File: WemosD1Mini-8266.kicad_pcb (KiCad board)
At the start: 2 copper layers, 79.9 x 51.8 mm, 54 parts, among them J1 Conn_01x02_Pin, J2 Screw_Terminal_01x10, J3 Conn_01x02_Pin, U1 PC817, U2 PC817, U3 PC817, U4 PC817, U5 WeMos_D1_mini, U6 ULN2003

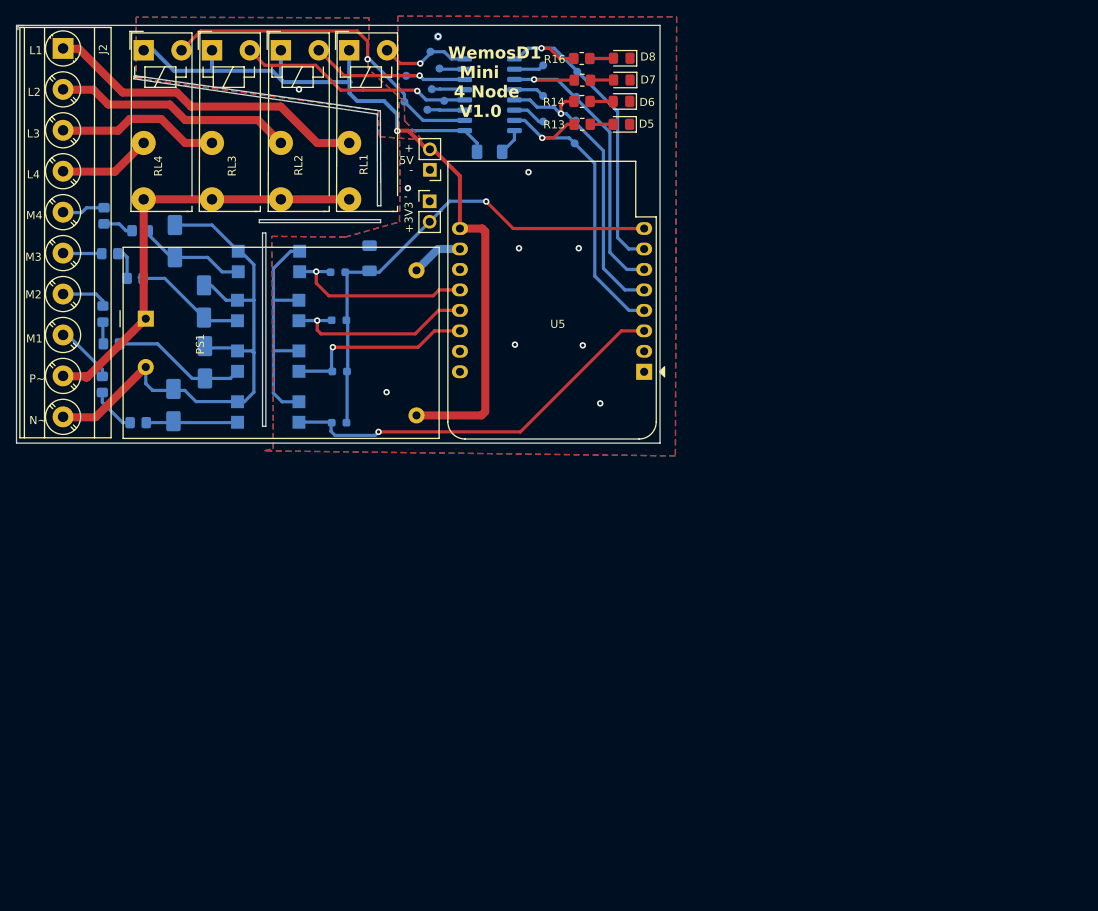
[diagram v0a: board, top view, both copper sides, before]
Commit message: Version 1.1
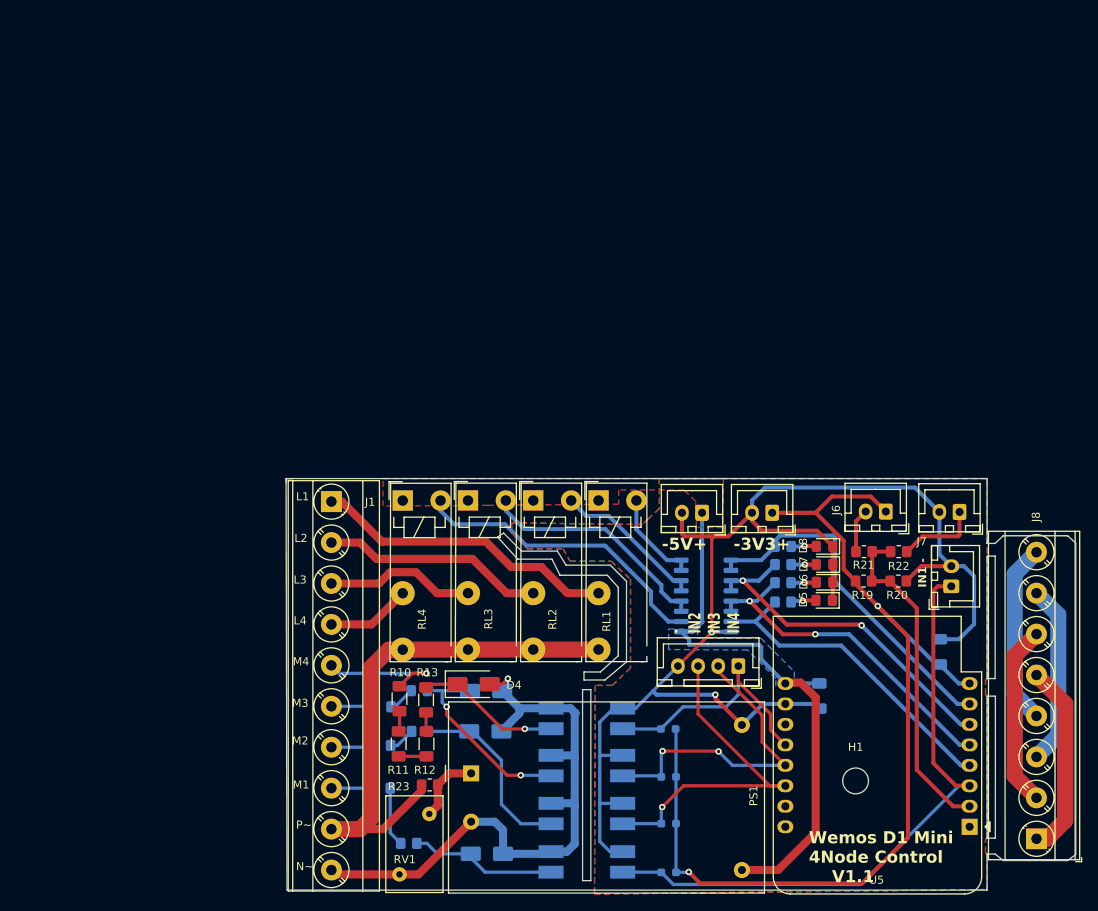
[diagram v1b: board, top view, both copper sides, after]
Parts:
- removed IJ1, IJ2, IJ3, IJ4, NCI1, NCI2, NCI3, NCR1, NCR2, NCR3, RJ1, RJ2, RJ3, RJ4: TestPoint, TestPoint:TestPoint_Pad_D1.0mm
- added H1: MountingHole, MountingHole:MountingHole_3.2mm_M3, F.Cu at (170.7, 137.5)
- added J4: Conn_01x04_Pin, Connector_JST:JST_XH_B4B-XH-A_1x04_P2.50mm_Vertical, F.Cu at (156.1, 123.3)
- added J5: Conn_01x02_Pin, Connector_JST:JST_XH_B2B-XH-A_1x02_P2.50mm_Vertical, F.Cu at (182.6, 113.4)
- added J6: Conn_01x02_Pin, Connector_JST:JST_XH_B2B-XH-A_1x02_P2.50mm_Vertical, F.Cu at (174.4, 104.1)
- added J7: Conn_01x02_Pin, Connector_JST:JST_XH_B2B-XH-A_1x02_P2.50mm_Vertical, F.Cu at (183.6, 104.1)
- added J8: Screw_Terminal_01x08, TerminalBlock_Phoenix:TerminalBlock_Phoenix_MKDS-3-8-5.08_1x08_P5.08mm_Horizontal, F.Cu at (193.1, 144.7)
- added R17: 480, Resistor_SMD:R_0805_2012Metric_Pad1.20x1.40mm_HandSolder, B.Cu at (161.7, 112.9)
- added R18: 480, Resistor_SMD:R_0805_2012Metric_Pad1.20x1.40mm_HandSolder, B.Cu at (161.7, 115.3)
- added R19: 10K, Resistor_SMD:R_0805_2012Metric_Pad1.20x1.40mm_HandSolder, F.Cu at (171.7, 112.7)
- added R20: 6.8K, Resistor_SMD:R_0805_2012Metric_Pad1.20x1.40mm_HandSolder, F.Cu at (176.0, 112.7)
- added R21: 2.2K, Resistor_SMD:R_0805_2012Metric_Pad1.20x1.40mm_HandSolder, F.Cu at (171.7, 109.1)
- added R22: 5.6K, Resistor_SMD:R_0805_2012Metric_Pad1.20x1.40mm_HandSolder, F.Cu at (176.0, 109.1)
- added R23: 0, Resistor_SMD:R_0805_2012Metric_Pad1.20x1.40mm_HandSolder, F.Cu at (117.8, 138.0)
- added RV1: Varistor, Varistor:RV_Disc_D12mm_W7.1mm_P7.5mm, F.Cu at (117.8, 141.6)
- D4: moved to F.Cu
- J1: value Conn_01x02_Pin -> Screw_Terminal_01x10; footprint Connector_PinHeader_2.54mm:PinHeader_1x02_P2.54mm_Vertical -> TerminalBlock_Phoenix:TerminalBlock_Phoenix_MKDS-3-10-5.08_1x10_P5.08mm_Horizontal
- J2: value Screw_Terminal_01x10 -> Conn_01x02_Pin; footprint TerminalBlock_Phoenix:TerminalBlock_Phoenix_MKDS-3-10-5.08_1x10_P5.08mm_Horizontal -> Connector_JST:JST_XH_B2B-XH-A_1x02_P2.50mm_Vertical
- J3: footprint Connector_PinHeader_2.54mm:PinHeader_1x02_P2.54mm_Vertical -> Connector_JST:JST_XH_B2B-XH-A_1x02_P2.50mm_Vertical
- R10, R11: value 180K -> 22K; footprint Resistor_SMD:R_0805_2012Metric_Pad1.20x1.40mm_HandSolder -> Resistor_SMD:R_1206_3216Metric_Pad1.30x1.75mm_HandSolder; moved to F.Cu
- R12: value 10K -> 22K; footprint Resistor_SMD:R_0603_1608Metric_Pad0.98x0.95mm_HandSolder -> Resistor_SMD:R_1206_3216Metric_Pad1.30x1.75mm_HandSolder; moved to F.Cu
- R13: value 480 -> 22K; footprint Resistor_SMD:R_0805_2012Metric_Pad1.20x1.40mm_HandSolder -> Resistor_SMD:R_1206_3216Metric_Pad1.30x1.75mm_HandSolder
- R14: value 480 -> 10K; footprint Resistor_SMD:R_0805_2012Metric_Pad1.20x1.40mm_HandSolder -> Resistor_SMD:R_0603_1608Metric_Pad0.98x0.95mm_HandSolder; moved to B.Cu
- R15, R16: moved to B.Cu
- U1, U2, U3, U4: footprint Package_DIP:DIP-4_W7.62mm_SMDSocket_SmallPads -> Package_DIP:DIP-4_W8.89mm_SMDSocket_LongPads
- moved J2 98.0 mm to (151.6, 104.2), turned to 180 degrees
- moved C1 86.0 mm to (181.1, 121.5)
- moved C2 79.0 mm to (166.2, 127.0), turned to -90 degrees
- moved R14 78.6 mm to (147.4, 131.1), turned to 180 degrees
- moved R13 74.0 mm to (117.4, 127.5), turned to 90 degrees
- moved R11 71.3 mm to (114.0, 132.9), turned to -90 degrees
- moved R10 70.3 mm to (114.1, 127.3)
- moved R9 69.9 mm to (147.5, 137.0)
- moved U5 69.4 mm to (184.8, 143.2)
- moved R6 69.4 mm to (147.5, 142.8)
- moved PS1 69.4 mm to (123.0, 136.6)
- moved R3 69.2 mm to (147.5, 148.9)
- moved U4 69.1 mm to (137.3, 129.8)
- moved U3 69.0 mm to (137.3, 135.6)
- moved U2 68.7 mm to (137.3, 141.6)
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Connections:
- C1 pad 1: /Voltage Sensing/+Vs -> +3.3V
- J1 pad 1: Earth -> /Load4
- J1 pad 2: +5V -> /Load3
- J2 pad 1: /Load4 -> +5V
- J2 pad 2: /Load3 -> Earth
- J3 pad 1: Earth -> +3.3V
- J3 pad 2: /Voltage Sensing/+Vs -> Earth
- PS1 pad 1: /AC/L -> /AC/L(P)
- R11 pad 2: Net-(D4-K) -> Net-(R11-Pad2)
- R12 pad 1: /Voltage Sensing/+Vs -> Net-(R11-Pad2)
- R12 pad 2: /Voltage Sensing/In4 -> Net-(R12-Pad2)
- R13 pad 1: /Relays/RL1 -> Net-(R12-Pad2)
- R13 pad 2: Net-(D5-A) -> Net-(D4-K)
- R14 pad 1: /Relays/RL2 -> +3.3V
- R14 pad 2: Net-(D6-A) -> /Voltage Sensing/In4
- R3 pad 1: /Voltage Sensing/+Vs -> +3.3V
- R6 pad 1: /Voltage Sensing/+Vs -> +3.3V
- R9 pad 1: /Voltage Sensing/+Vs -> +3.3V
- U5 pad 2: unconnected-(U5-A0-Pad2) -> Net-(U5-A0)
- U5 pad 8: /Voltage Sensing/+Vs -> +3.3V
- U6 pad 11: Net-(U6-O6) -> Net-(U6-O5)
- U6 pad 13: Net-(U6-O4) -> Net-(U6-O3)
- U6 pad 15: Net-(U6-O2) -> Net-(U6-O1)
- U6 pad 2: Net-(U6-I2) -> /Relays/RL4
- U6 pad 4: Net-(U6-I4) -> /Relays/RL3
- U6 pad 6: Net-(U6-I6) -> /Relays/RL2
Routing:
- net Earth: track 39.4 -> 167.3 mm, vias 9 -> 2
- net +3.3V: track 0.00 -> 125.7 mm, vias 0 -> 2
- net /Voltage Sensing/+Vs: track 61.1 -> 0.00 mm, vias 1 -> 0
- net Net-(U5-A0): track 0.00 -> 41.5 mm
- net +5V: track 110.7 -> 70.2 mm, vias 2 -> 0
- net /Voltage Sensing/In1: track 49.5 -> 78.3 mm, vias 1 -> 0
- net Net-(J8-Pin_1): track 0.00 -> 24.0 mm
- net Net-(J8-Pin_3): track 0.00 -> 22.6 mm
- net Net-(J8-Pin_4): track 0.00 -> 22.6 mm
- net Net-(J8-Pin_2): track 0.00 -> 22.6 mm
- net /Voltage Sensing/In2: track 23.8 -> 43.8 mm
- net /Voltage Sensing/In3: track 24.3 -> 39.9 mm, vias 1 -> 2
- net /M4: track 5.20 -> 16.2 mm, vias 0 -> 1
- net Net-(D3-K): track 14.0 -> 24.6 mm, vias 0 -> 2
- net Net-(J7-Pin_1): track 0.00 -> 10.2 mm
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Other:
- board size 79.9 x 51.8 mm -> 98 x 51.1 mm
- board text added: "- IN2 IN3 IN4"
- board text added: "-3V3+"
- board text added: "-5V+"
- board text added: "IN1 -"
- board text added: "Wemos D1 Mini 4Node Control V1.1"
- board text removed: "+"
- board text removed: "-"
- board text removed: "3V3"
- board text removed: "5V"
- board text removed: "CAUTION: High Voltage"
- board text removed: "Wemos D1 Mini 4Node Control V1.0"
- board text removed: "WemosD1 Mini 4 Node V1.0"
